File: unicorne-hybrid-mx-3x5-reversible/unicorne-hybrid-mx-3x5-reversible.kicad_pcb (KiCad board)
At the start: 2 copper layers, 114.7 x 91.4 mm, 84 parts, among them J1 MJ-4PP-9, J2 Nice!View, J3 Conn_01x02, J4 Conn_01x03, SW1 SW_MX_HS, SW10 SW_MX_HS, SW11 SW_MX_HS, SW12 SW_MX_HS, SW13 SW_MX_HS, SW14 SW_MX_HS, SW15 SW_MX_HS, SW16 SW_MX_HS, SW17 SW_MX_HS, SW18 SW_MX_HS, SW2 SW_MX_HS, SW3 SW_MX_HS, SW4 SW_MX_HS, SW5 SW_MX_HS, SW6 SW_MX_HS, SW7 SW_MX_HS, SW8 SW_MX_HS, SW9 SW_MX_HS, U1 ProMicro-ish

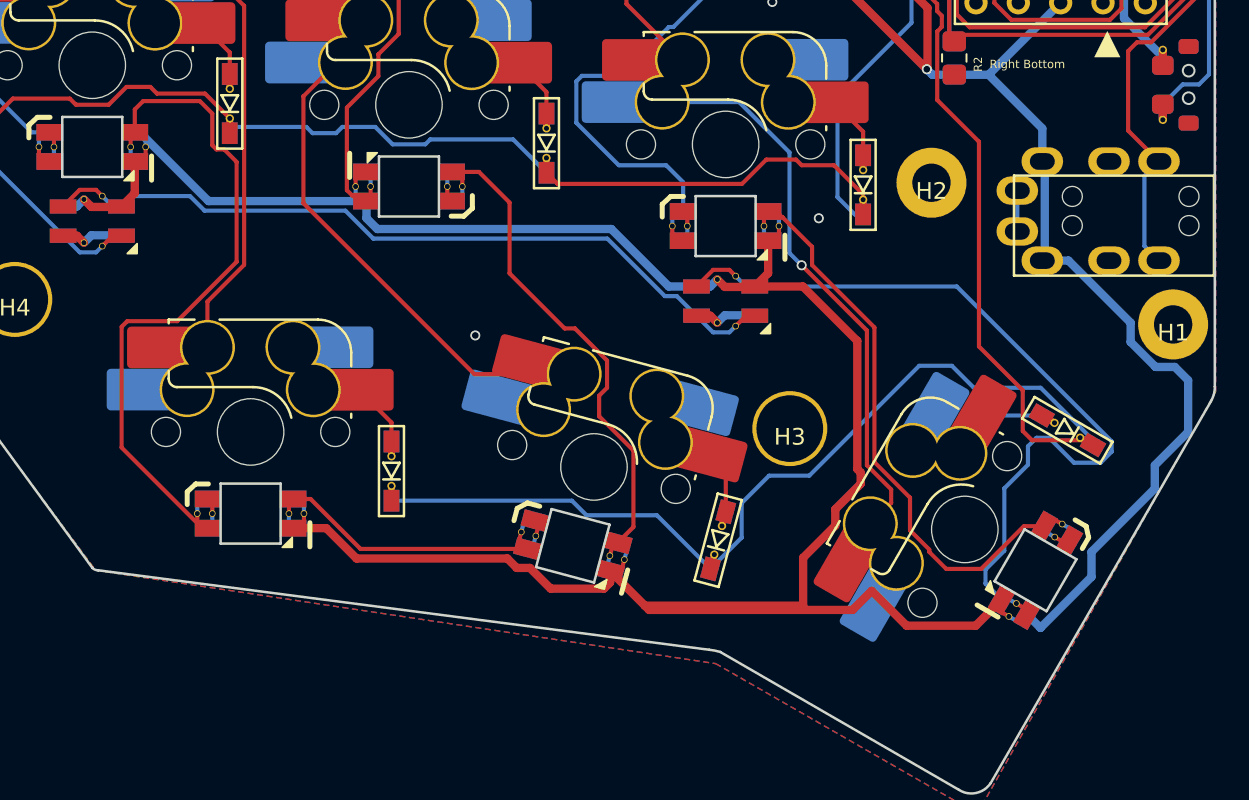
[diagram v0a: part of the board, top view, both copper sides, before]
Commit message: hybrid
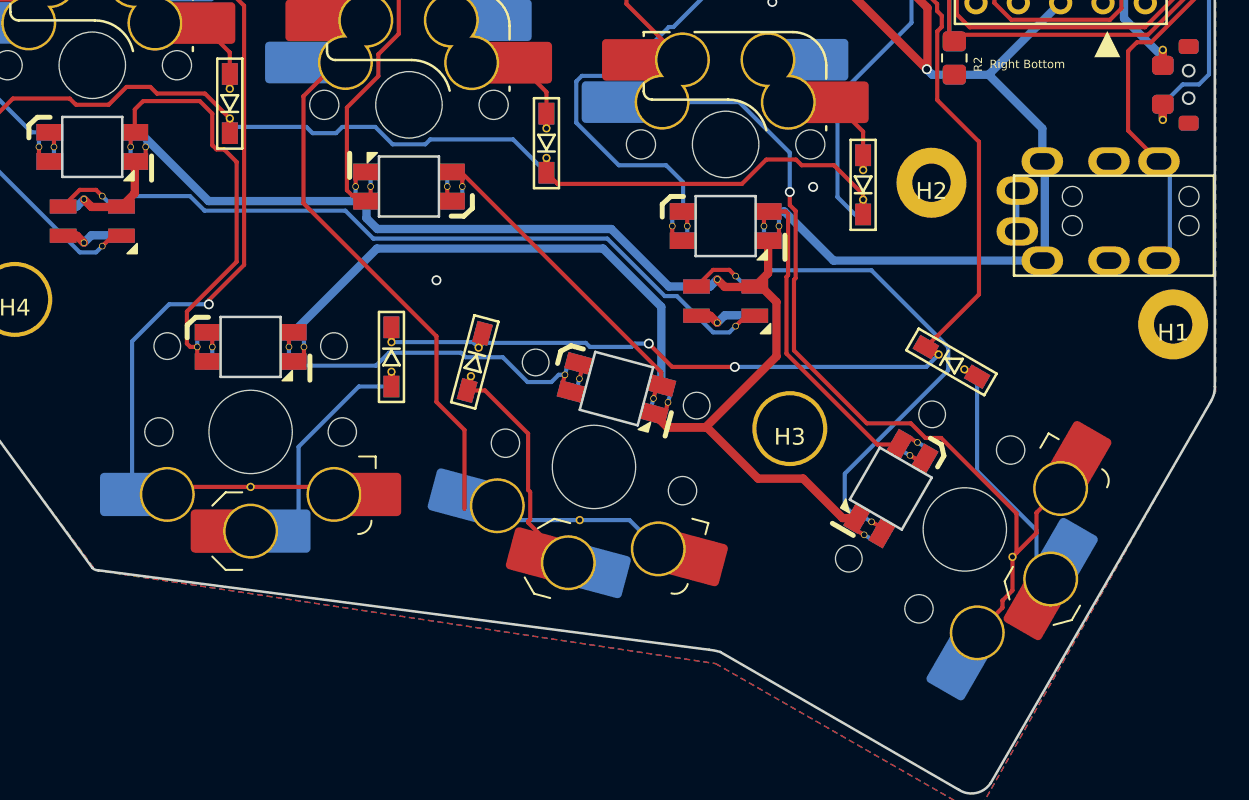
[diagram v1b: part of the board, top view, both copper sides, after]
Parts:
- SW16, SW17: value SW_MX_HS -> SW_CHOC_HS; footprint KBD_PARTS:SW_MX_HS_1u_reversible -> KBD_PARTS:SW_choc_v1_v2_HS_1u_reversible
- SW18: value SW_MX_HS -> SW_CHOC_HS; footprint KBD_PARTS:SW_MX_HS_1.5u_reversible -> KBD_PARTS:SW_choc_v1_v2_HS_1u_reversible
- moved D17 18.1 mm to (150.3, 126.6), turned to -105 degrees
- moved L16 10.00 mm to (136.8, 125.7)
- moved L18 9.97 mm to (175.3, 134.2)
- moved L17 9.79 mm to (158.8, 128.2)
- moved D18 8.07 mm to (178.9, 126.6), turned to -30 degrees
- moved D16 6.85 mm to (145.3, 126.3), turned to -90 degrees
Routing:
- net VCC: track 562.3 -> 524.1 mm
- net row3: track 115.6 -> 89.2 mm, vias 1 -> 3
- net col2: track 178.6 -> 201.1 mm, vias 1 -> 2
- net col4: track 130.5 -> 148.1 mm
- net Net-(L13-DIN): track 38.9 -> 23.2 mm
- net Net-(L18-DIN): track 46.5 -> 30.9 mm
- net Net-(L15-DIN): track 32.6 -> 18.7 mm
- net col3: track 140.9 -> 153.5 mm
- net Net-(D17-A): track 2.46 -> 13.9 mm
- net Net-(L14-DOUT): track 28.9 -> 18.4 mm
- net Net-(D16-A): track 3.92 -> 12.5 mm
- net Net-(D18-A): track 5.85 -> 14.0 mm
- net Net-(L16-DIN): track 15.3 -> 17.6 mm
